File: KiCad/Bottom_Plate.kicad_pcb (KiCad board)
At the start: 2 copper layers, 140 x 91.2 mm, 11 parts

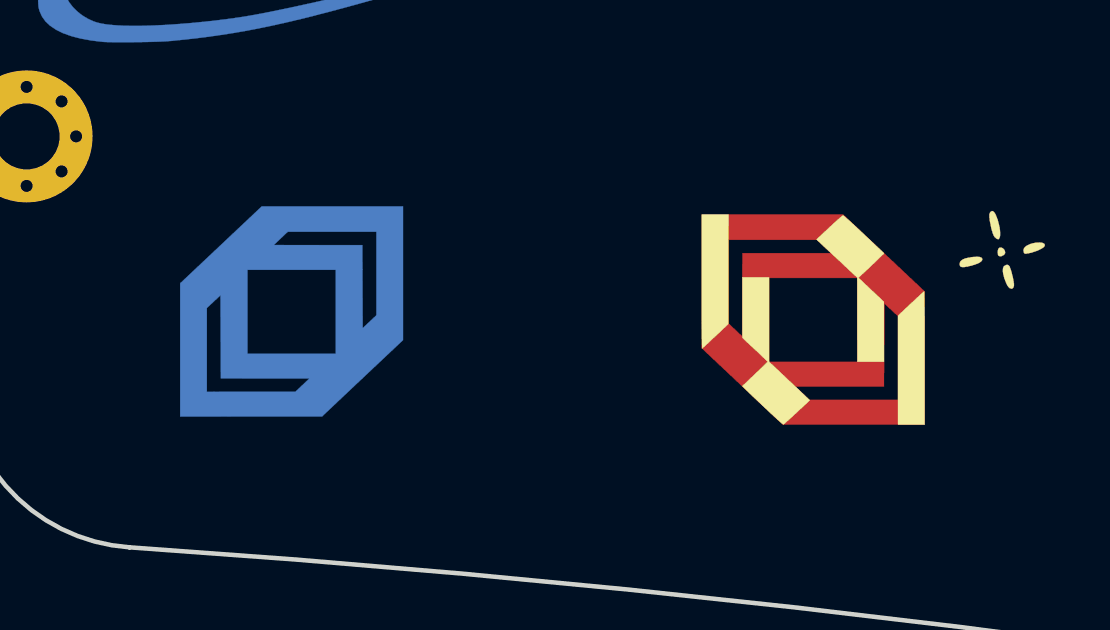
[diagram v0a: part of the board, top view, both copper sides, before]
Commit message: wip
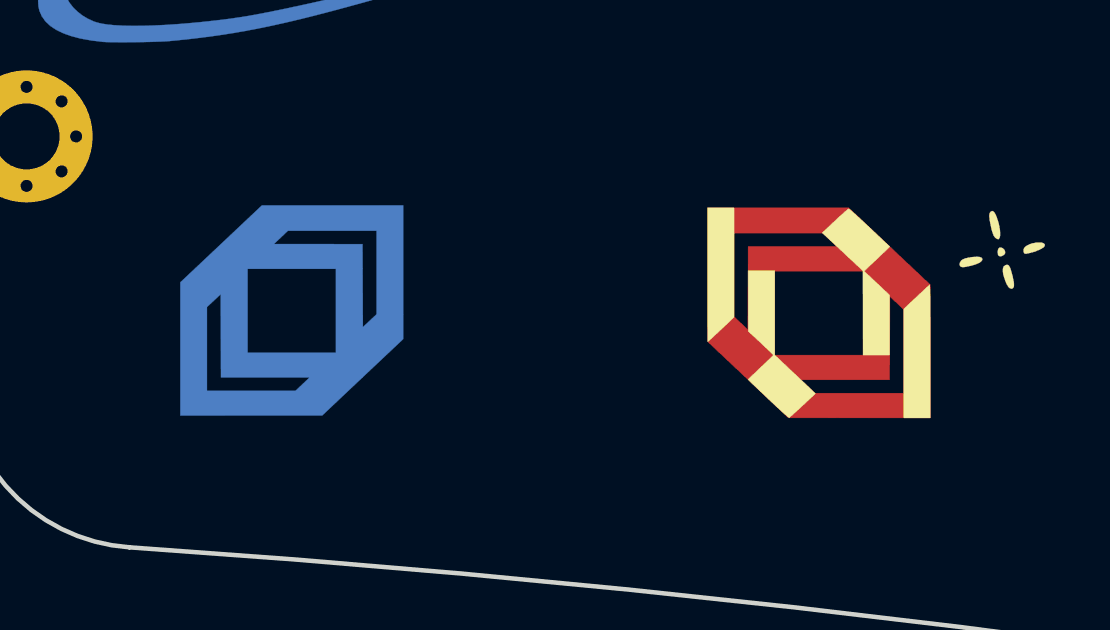
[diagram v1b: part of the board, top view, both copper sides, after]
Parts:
- removed the ? at (179.4, 182.0)
- removed the ? at (155.1, 181.7)
- added ?: , clipboard:9b0fb884-d604-4a4e-b347-07e1aeb927c7, F.Cu at (174.2, 181.9)
- added ?: , clipboard:9b0fb884-d604-4a4e-b347-07e1aeb927c7, B.Cu at (160.5, 181.8)
